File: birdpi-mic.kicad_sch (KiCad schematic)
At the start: 6 parts, among them U1 OPA1612AID, U2 TLE2426xD

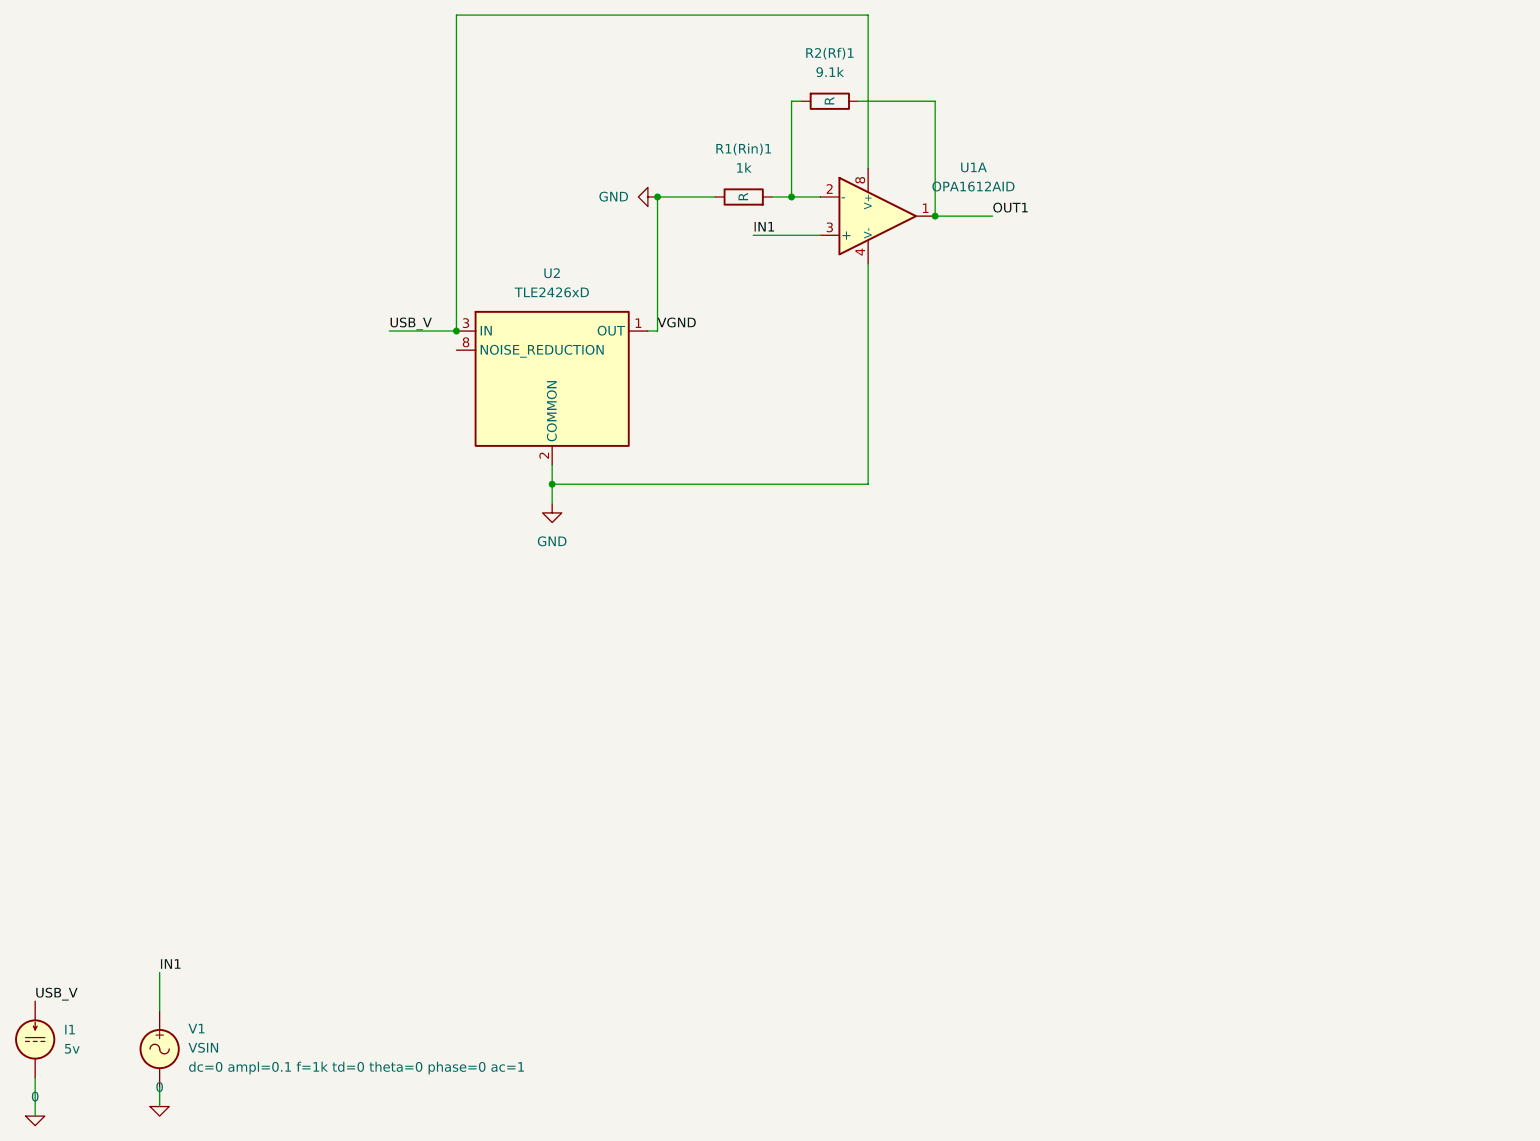
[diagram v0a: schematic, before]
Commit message: Now with a working simulation!
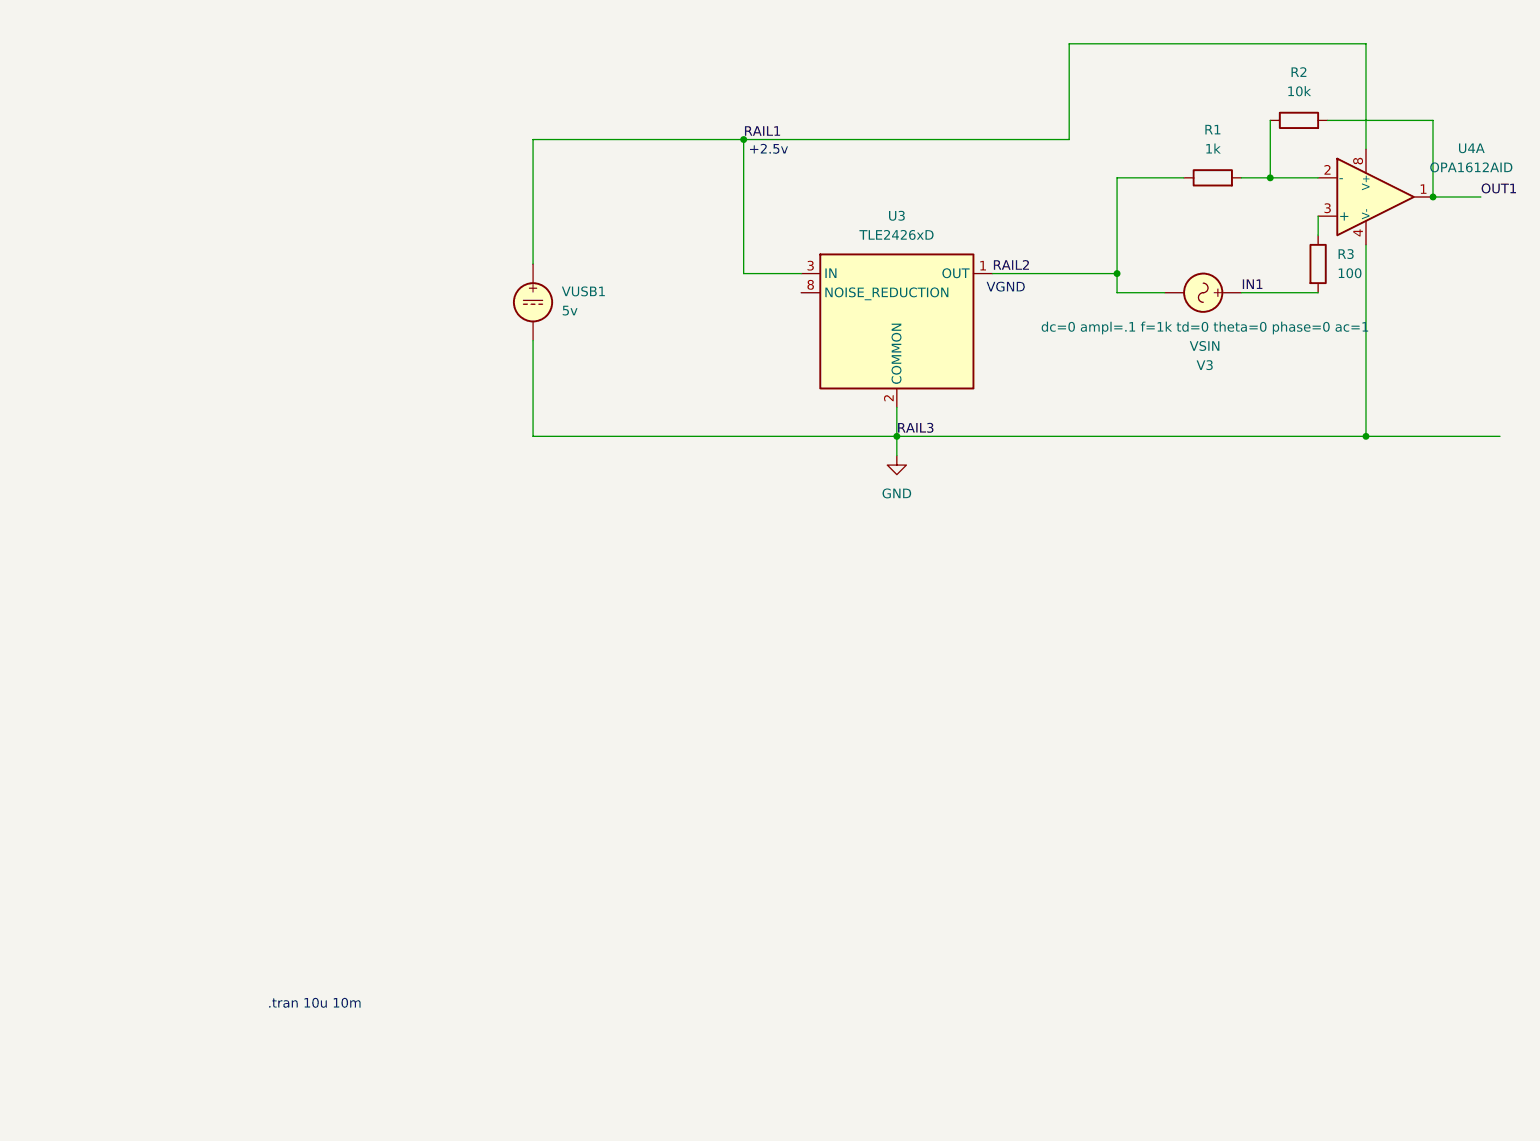
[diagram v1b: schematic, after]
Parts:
- removed I1: 5v, symbol Simulation_SPICE:IDC
- removed R1(Rin)1: 1k, symbol Device:R
- removed R2(Rf)1: 9.1k, symbol Device:R
- removed U1: OPA1612AID, PCM_Package_SO_AKL:SO-8_3.9x4.9mm_P1.27mm, symbol PCM_Amplifier_Operational_AKL:OPA1612AID
- removed U2: TLE2426xD, Package_SO:SOIC-8_3.9x4.9mm_P1.27mm, symbol Reference_Voltage:TLE2426xD
- removed V1: VSIN, symbol Simulation_SPICE:VSIN
- added R1: 1k, symbol Device:R
- added R2: 10k, symbol Device:R
- added R3: 100, symbol Device:R
- added U3: TLE2426xD, Package_SO:SOIC-8_3.9x4.9mm_P1.27mm, symbol Reference_Voltage:TLE2426xD
- added U4: OPA1612AID, PCM_Package_SO_AKL:SO-8_3.9x4.9mm_P1.27mm, symbol PCM_Amplifier_Operational_AKL:OPA1612AID
- added V3: VSIN, symbol Simulation_SPICE:VSIN
- added VUSB1: 5v, symbol Simulation_SPICE:VDC
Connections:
- net GND: now also U3.2 (COMMON), U4.4 (V-), VUSB1.2
- net IN1: now also R3.2, V3.1
- net OUT1: now also R2.2, U4.1
- new net: R1.2, R2.1, U4.2 (-)
- new net: R3.1, U4.3 (+)
- new net RAIL1: U3.3 (IN), U4.8 (V+), VUSB1.1
- new net RAIL2: R1.1, U3.1 (OUT), V3.2
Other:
- note added: "+2.5v"
- note added: ".tran 10u 10m"
- note added: "VGND"
